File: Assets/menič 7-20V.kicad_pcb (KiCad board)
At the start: 2 copper layers, 50 x 35 mm, 13 parts, among them U1 L7805

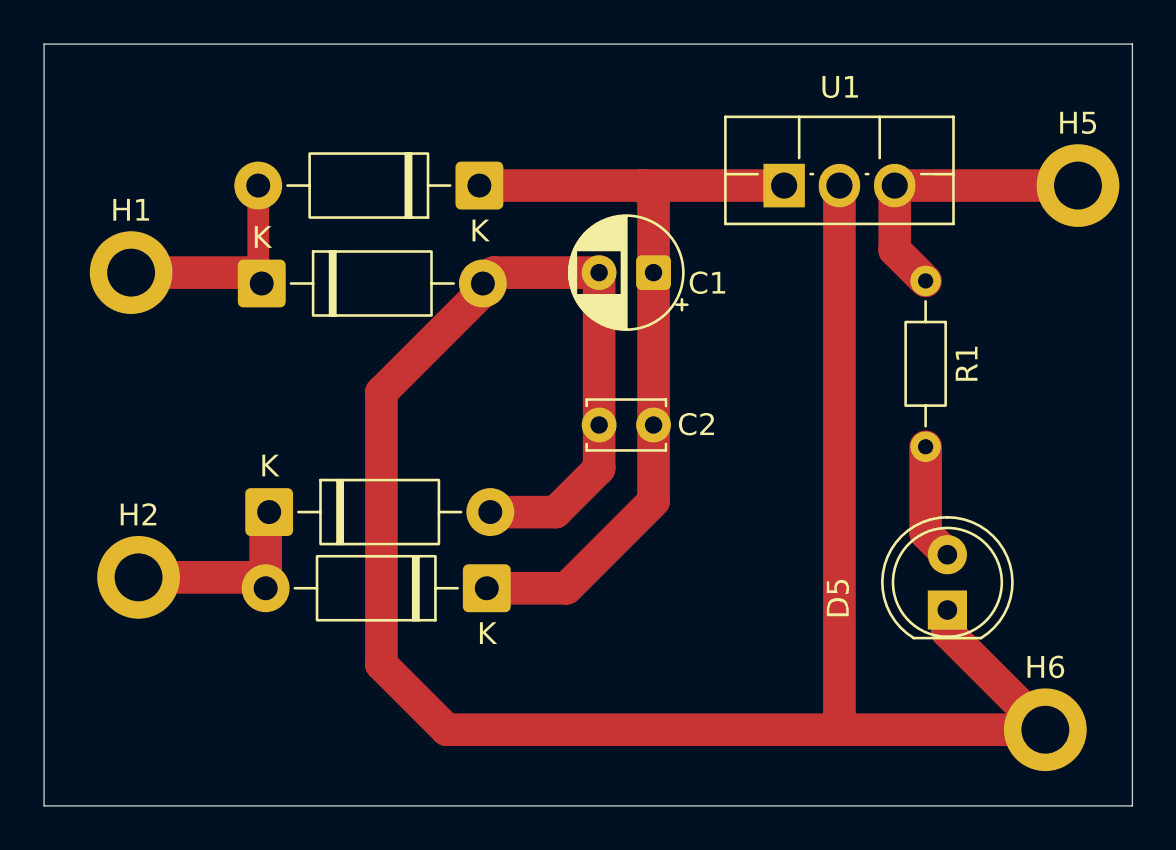
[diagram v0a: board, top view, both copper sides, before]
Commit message: Add files via upload
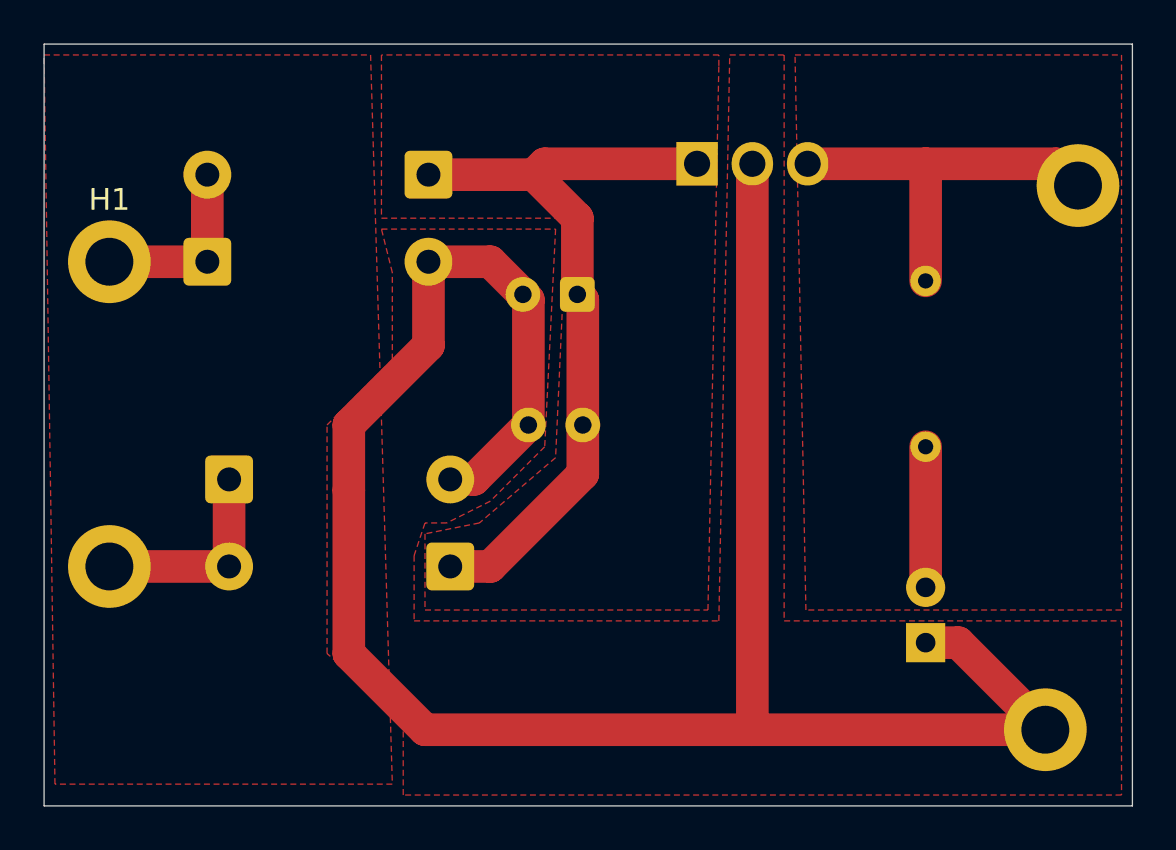
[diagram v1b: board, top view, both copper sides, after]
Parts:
- C1, C2, D1, D2, D3, D4, D5, H2, H5, H6, R1, U1: moved to B.Cu
- moved U1 4.12 mm to (125.5, 110.5)
- moved C1 3.64 mm to (120.0, 116.5)
- moved C2 3.25 mm to (117.8, 122.5)
- moved D2 2.69 mm to (103.0, 115.0)
- moved D1 2.39 mm to (113.2, 111.0)
- moved D3 2.37 mm to (104.0, 125.0)
- moved D4 1.96 mm to (114.2, 129.0)
- moved D5 1.80 mm to (136.0, 132.5)
- moved H2 1.43 mm to (98.5, 129.0), turned to 180 degrees
- moved H1 1.12 mm to (98.5, 115.0)
- turned H5 to 180 degrees
- turned H6 to 180 degrees
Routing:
- net Net-(U1-OUT): track 13.5 -> 18.2 mm
- net Net-(D1-K): track 38.0 -> 35.1 mm
- net Net-(D1-A): track 11.0 -> 8.50 mm
- net Net-(D2-A): track 103.9 -> 101.8 mm
- net Net-(D5-A): track 5.37 -> 6.46 mm
- added copper zone on F.Cu, net Net-(D1-A)
- added copper zone on F.Cu, net Net-(D1-K)
- added copper zone on F.Cu, net Net-(D2-A)
- added copper zone on F.Cu, net Net-(U1-OUT)
